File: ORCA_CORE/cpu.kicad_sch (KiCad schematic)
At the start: 25 parts, among them J10 Raspberry_Pi_2_3, J11 wheel_left, J8 wheel_front, J9 wheel_right, Q1 BSS138, Q2 BSS138, Q8 BSS138, U14 BNO055, U2 PCA9685PW_Q900_118

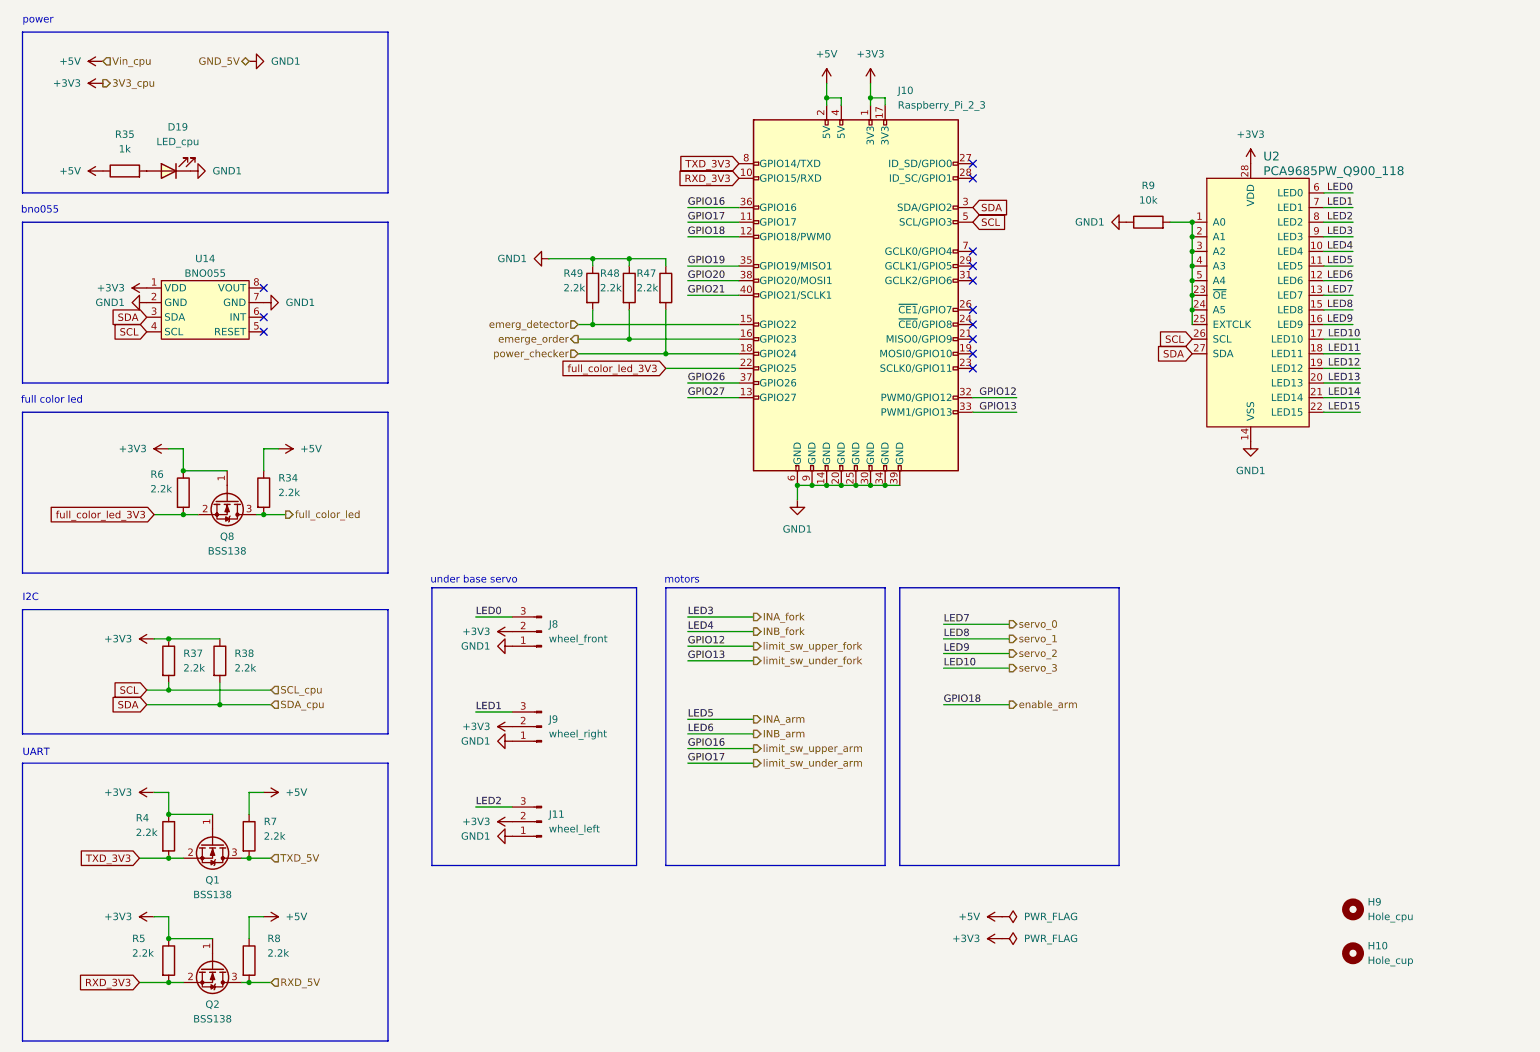
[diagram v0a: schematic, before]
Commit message: almost completed CORE
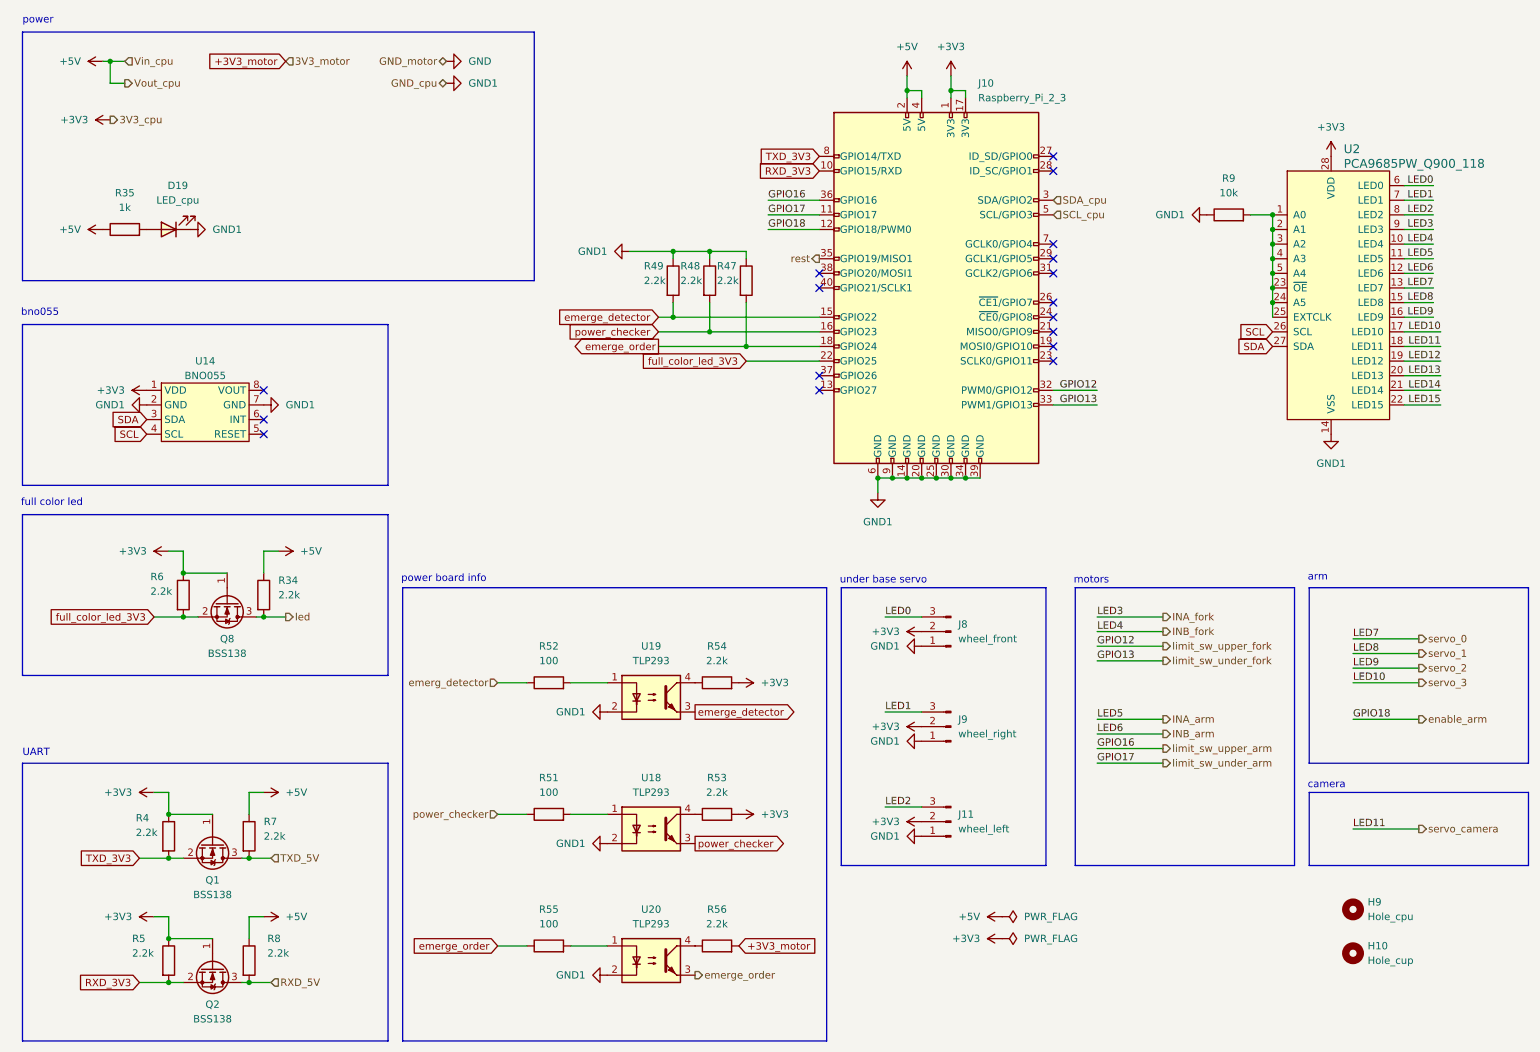
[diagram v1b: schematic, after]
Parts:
- removed R37, R38: 2.2k, Resistor_SMD:R_0603_1608Metric_Pad0.98x0.95mm_HandSolder, symbol Device:R
- added R51, R52, R55: 100, symbol Device:R
- added R53, R54, R56: 2.2k, symbol Device:R
- added U18, U19, U20: TLP293, Package_SO:SOIC-4_4.55x2.6mm_P1.27mm, symbol Isolator:TLP293
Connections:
- net +3V3: now also R53.2, R54.2
- net GND1: now also U18.2, U19.2, U20.2
- net SCL: no longer J10.5 (SCL/GPIO3)
- net SDA: no longer J10.3 (SDA/GPIO2)
- net emerg_detector: now also R52.1; no longer J10.15 (GPIO22), R49.2
- net emerge_order: now also J10.18 (GPIO24), R47.2, R55.1, U20.3; no longer J10.16 (GPIO23), R48.2
- net power_checker: now also J10.16 (GPIO23), R48.2, R51.1, U18.3; no longer J10.18 (GPIO24), R47.2
- net GPIO19 renamed rest
- net GPIO20: no longer names the net of J10.38 (GPIO20/MOSI1)
- net GPIO21: no longer names the net of J10.40 (GPIO21/SCLK1)
- net GPIO26: no longer names the net of J10.37 (GPIO26)
- net GPIO27: no longer names the net of J10.13 (GPIO27)
- net LED11 renamed servo_camera
- net full_color_led renamed led
- new net: R52.2, U19.1
- new net: R54.1, U19.4
- new net: R51.2, U18.1
- new net: R53.1, U18.4
- new net: R55.2, U20.1
- new net: R56.1, U20.4
- new net +3V3_motor: R56.2
- new net SCL_cpu: J10.5 (SCL/GPIO3)
- new net SDA_cpu: J10.3 (SDA/GPIO2)
- new net emerge_detector: J10.15 (GPIO22), R49.2, U19.3
- no-connect marks 13 -> 17
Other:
- note added: "arm"
- note added: "camera"
- note added: "power board info"
- note removed: "I2C"
- moved on the sheet: D19, J10, J11, J8, J9, Q8, R34, R35, R47, R48, R49, R6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
